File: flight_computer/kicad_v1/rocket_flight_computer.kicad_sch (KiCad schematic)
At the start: 17 parts, among them U2 Teensy4.1, U3 BMI088, U5 BMP280

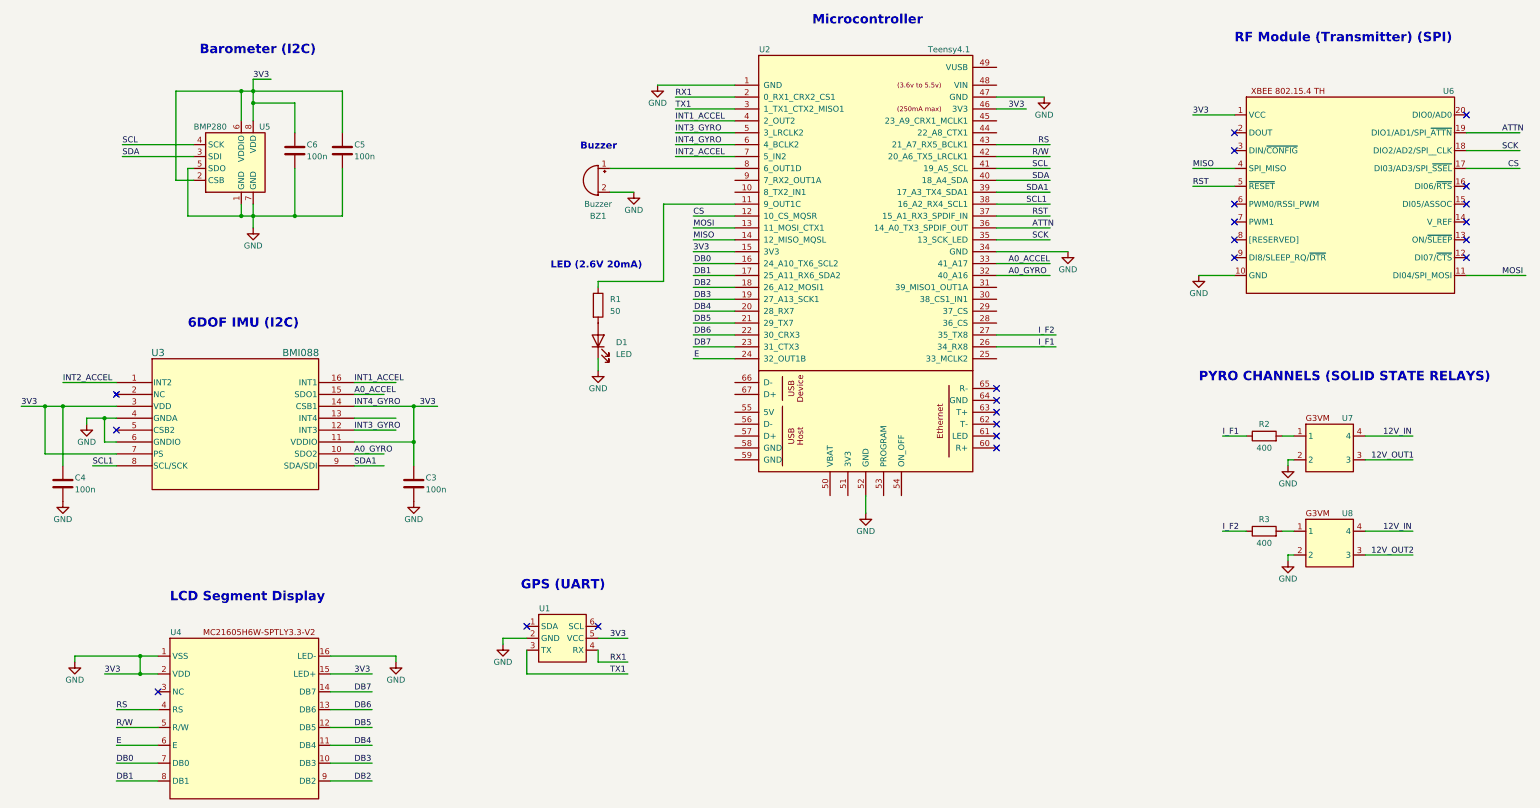
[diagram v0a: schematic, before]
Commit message: noisy c model
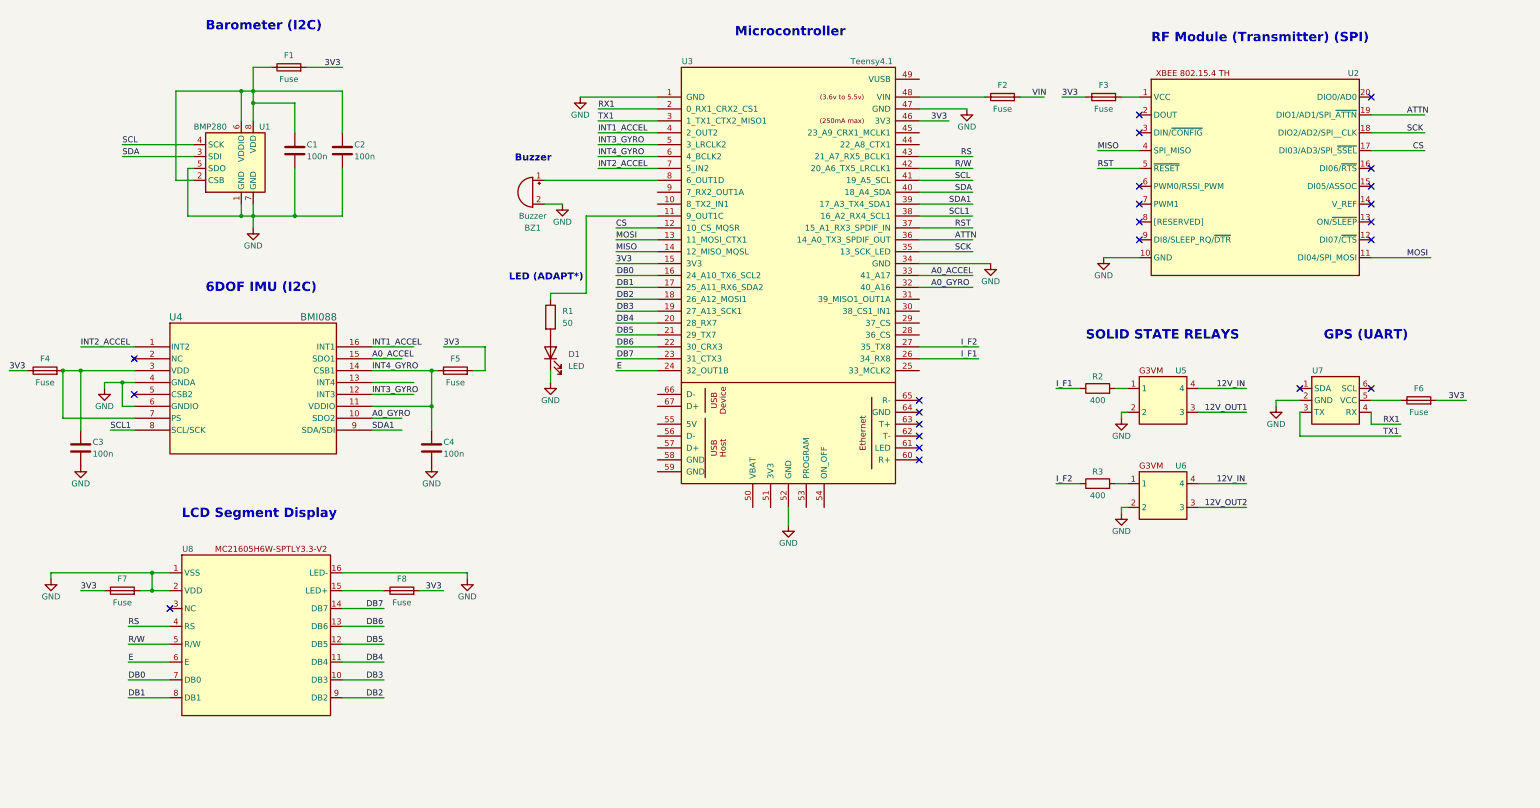
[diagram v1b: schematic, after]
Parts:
- added F1, F2, F3, F4, F5, F6, F7, F8: Fuse, symbol Device:Fuse
- renumbered C6 to C1, C5 to C2, C4 to C3, C3 to C4, U5 to U1, U6 to U2, U2 to U3, U3 to U4, U7 to U5, U8 to U6, U1 to U7, U4 to U8
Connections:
- net GND: now also F7.2; no longer C1.1, C2.1, C3.1, C4.1, U1.2 (CSB), U1.6 (VDDIO), U1.8 (VDD), U2.1 (VCC), U3.15 (3V3), U3.46 (3V3), U3.6 (4_BCLK2), U4.11 (VDDIO), U4.14 (CSB1), U4.3 (VDD), U4.7 (PS), U7.5 (VCC), U8.15 (LED+)
- net at U3.48 (VIN): now also F2.1
- new net: C3.1, F4.2, U4.3 (VDD), U4.7 (PS)
- new net: C1.1, C2.1, F1.1, U1.2 (CSB), U1.6 (VDDIO), U1.8 (VDD)
- new net: F3.2, U2.1 (VCC)
- new net: F8.1, U8.15 (LED+)
- new net: F6.1, U7.5 (VCC)
- new net 3V3: F1.2, F3.1, F4.1, F5.2, F6.2, F7.1, F8.2, U3.15 (3V3), U3.46 (3V3)
- new net INT4_GYRO: C4.1, F5.1, U3.6 (4_BCLK2), U4.11 (VDDIO), U4.14 (CSB1)
- new net VIN: F2.2
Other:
- note added: "LED (ADAPT*)"
- note added: "SOLID STATE RELAYS"
- note removed: "LED (2.6V 20mA)"
- note removed: "PYRO CHANNELS (SOLID STATE RELAYS)"
- moved on the sheet: BZ1, C3, C4, D1, R1, R2, R3, U2, U3, U4, U5, U6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
